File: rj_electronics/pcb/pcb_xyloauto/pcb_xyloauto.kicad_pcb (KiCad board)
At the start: 2 copper layers, 180.3 x 36.2 mm, 13 parts, among them J1 Conn_01x08_Pin, J2 Conn_01x08_Pin, J3 Conn_01x02_Pin, J4 Barrel_Jack, U1 Sparkfun_Pro_Micro, U2 ULN2803A, U3 LM317_TO-220

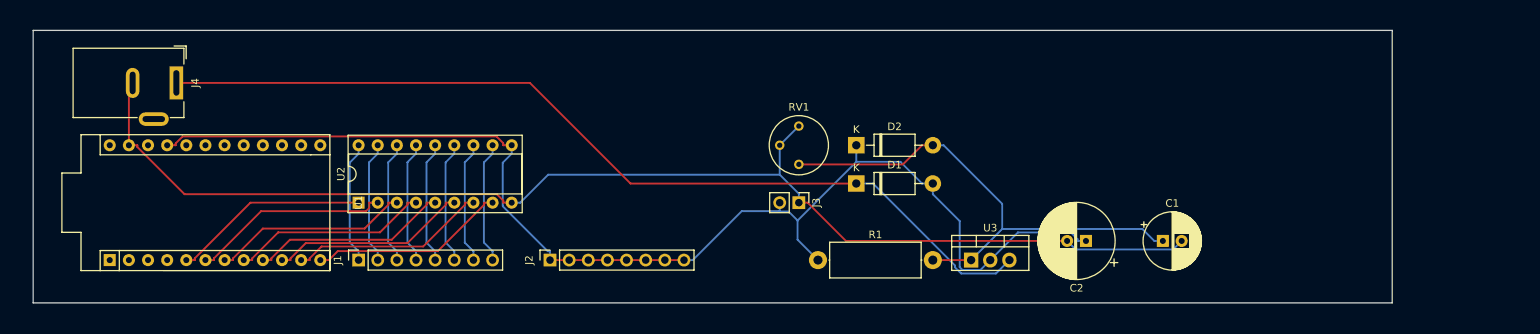
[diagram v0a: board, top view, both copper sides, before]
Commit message: nc
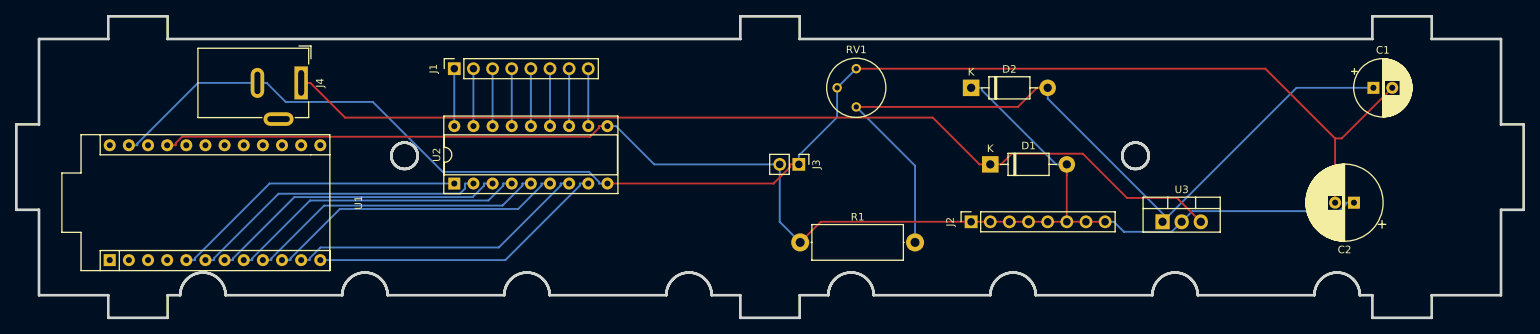
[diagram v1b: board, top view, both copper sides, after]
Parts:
- moved J2 56.1 mm to (157.5, 137.2)
- moved C2 35.9 mm to (208.3, 134.6)
- moved C1 34.5 mm to (210.9, 119.4)
- moved J1 28.4 mm to (88.9, 116.8)
- moved U3 25.9 mm to (182.9, 137.2)
- moved D1 18.0 mm to (160.0, 129.5)
- moved D2 17.0 mm to (157.5, 119.4)
- moved J4 16.6 mm to (68.6, 118.7)
- moved U2 13.0 mm to (88.9, 132.1)
- moved RV1 10.8 mm to (142.2, 121.9)
- moved J3 5.08 mm to (134.6, 129.5)
- moved R1 3.33 mm to (134.8, 139.9)
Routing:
- net Net-(D2-A): track 67.5 -> 106.8 mm
- net GND: track 165.7 -> 201.5 mm
- net VOUT: track 165.8 -> 197.9 mm
- net Net-(U1-D7): track 26.3 -> 40.1 mm
- net Net-(U1-~D9/A9): track 26.2 -> 39.9 mm
- net Net-(U1-~D6/A7): track 26.3 -> 40.1 mm
- net Net-(U1-~D5): track 26.3 -> 40.1 mm
- net Net-(U1-D2): track 26.2 -> 39.9 mm
- net Net-(U1-D8/A8): track 26.3 -> 40.1 mm
- net Net-(U1-D4/A6): track 26.3 -> 40.1 mm
- net Net-(U1-~D3): track 26.6 -> 40.3 mm
- net Net-(J1-Pin_1): track 16.2 -> 7.62 mm
- net Net-(J1-Pin_8): track 16.2 -> 7.62 mm
- net Net-(J1-Pin_7): track 16.2 -> 7.62 mm
- net Net-(J1-Pin_6): track 16.2 -> 7.62 mm
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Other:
- board size 180.3 x 36.2 mm -> 200 x 40 mm
